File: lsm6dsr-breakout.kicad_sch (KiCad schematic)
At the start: 15 parts, among them CN1 AFC10-S04QCA-00, CN2 AFC10-S04QCA-00, J1 Conn_01x06_Pin, J2 Conn_01x04_Pin, U1 LSM6DSRTR

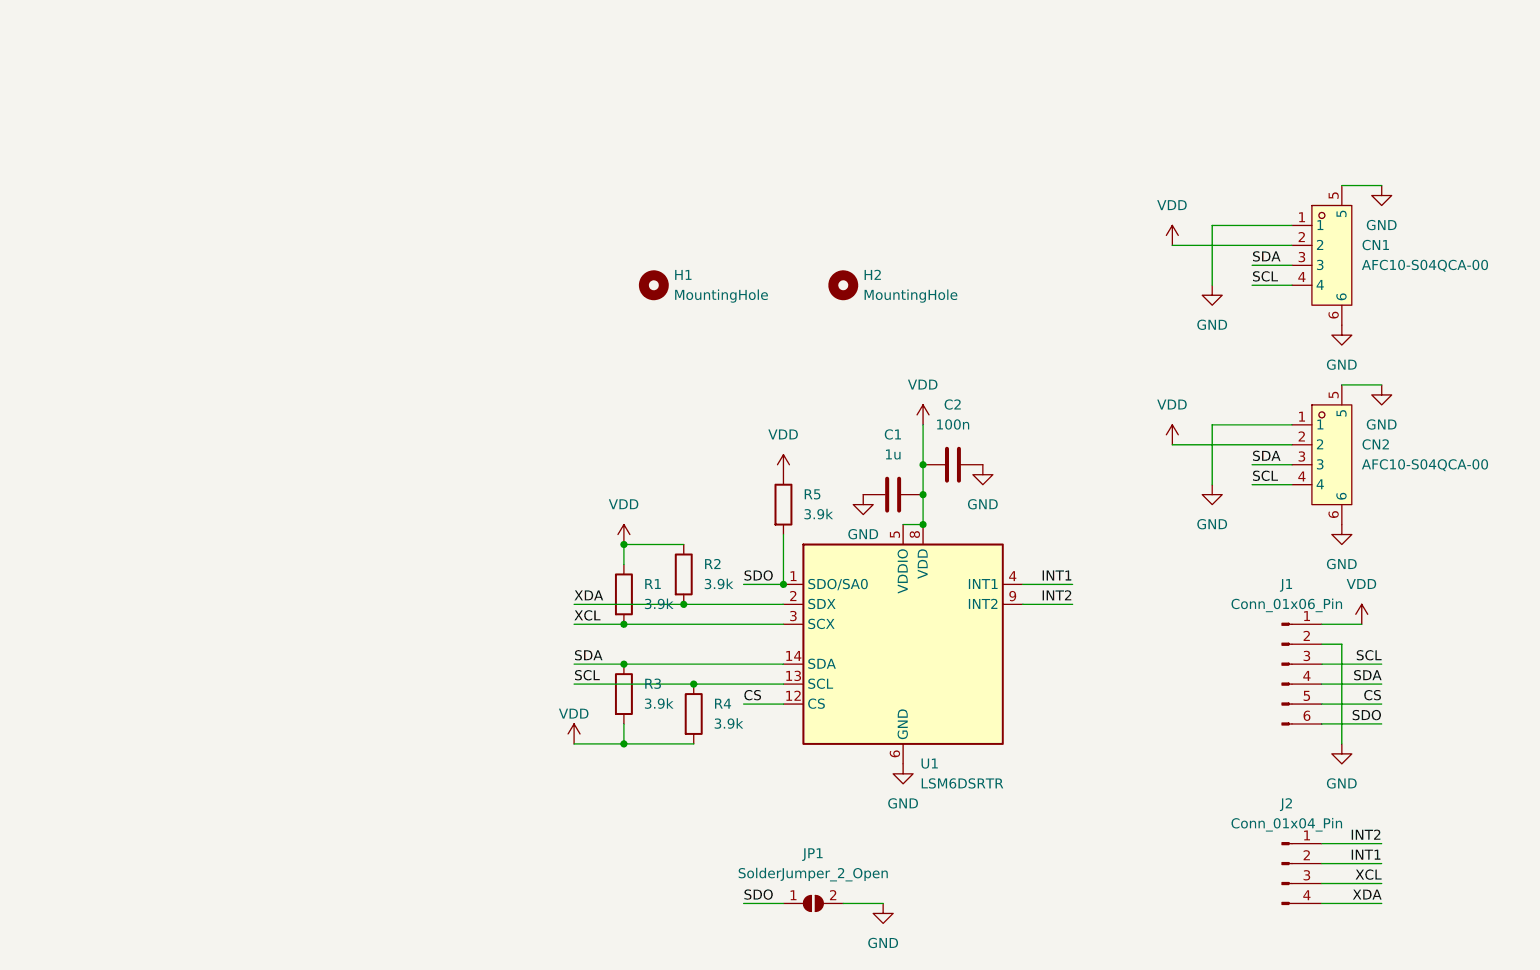
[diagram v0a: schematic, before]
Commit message: beautify schematic
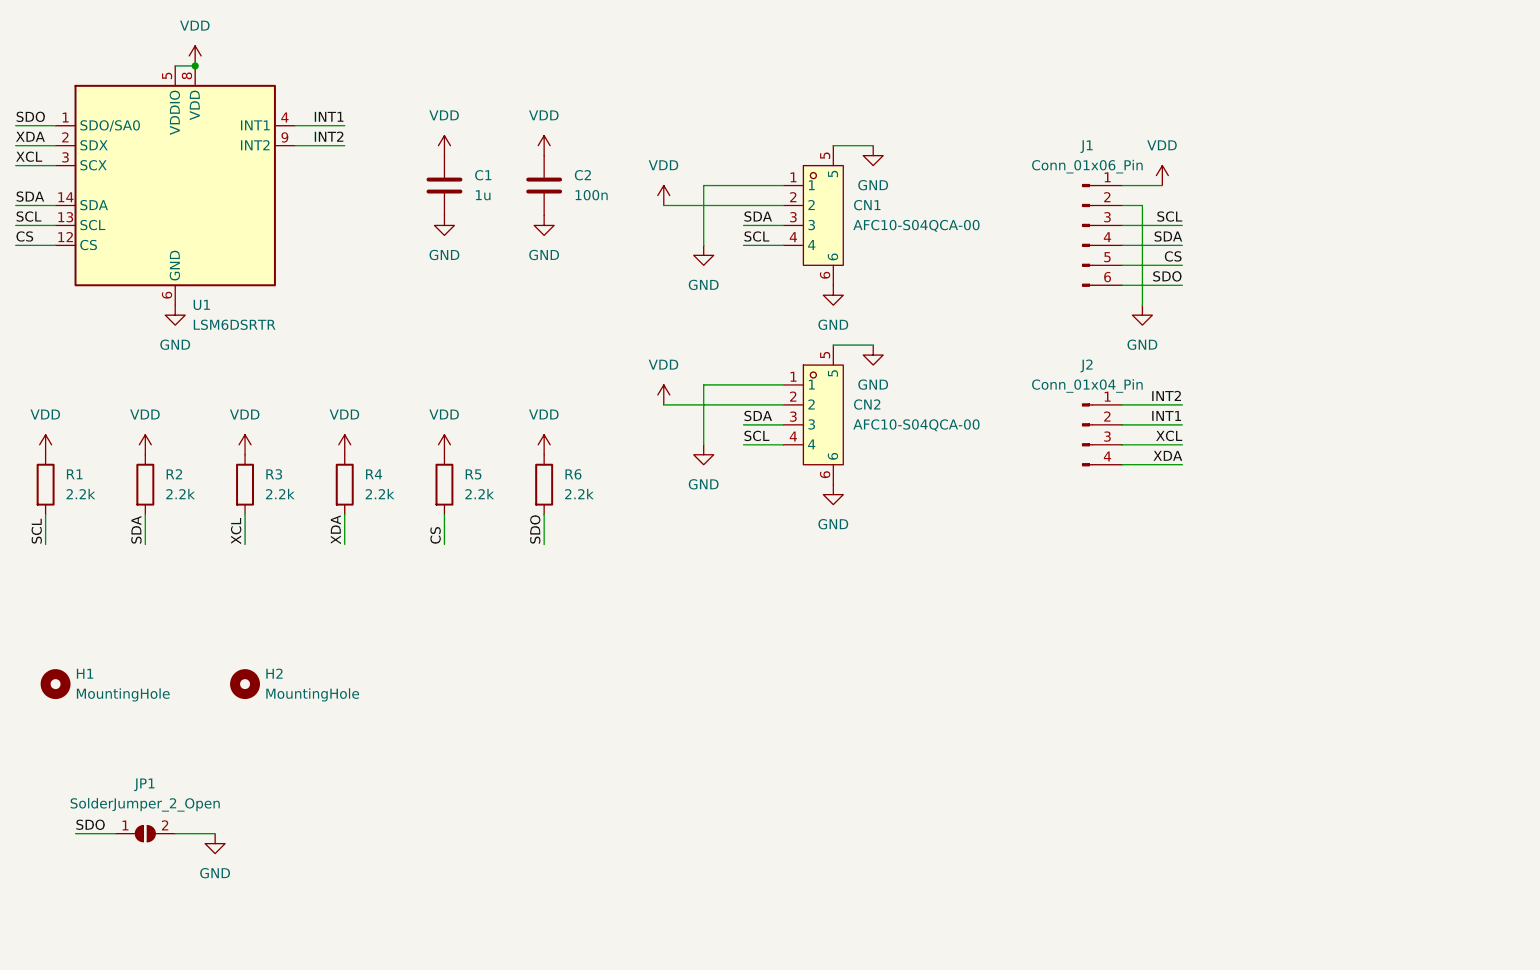
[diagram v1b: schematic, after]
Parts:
- added R6: 2.2k, Resistor_SMD:R_0402_1005Metric, symbol Device:R
- R1, R2, R3, R4, R5: value 3.9k -> 2.2k
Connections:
- net CS: now also R5.2
- net GND: now also C1.2; no longer C1.1
- net SCL: now also R1.2; no longer R4.1
- net SDA: now also R2.2; no longer R3.1
- net SDO: now also R6.2; no longer R5.2
- net VDD: now also C1.1, R3.1, R4.1, R6.1; no longer C1.2, R3.2, R4.2
- net XCL: now also R3.2; no longer R1.2
- net XDA: now also R4.2; no longer R2.2
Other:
- moved on the sheet: CN1, CN2, H1, H2, J1, J2, JP1, U1
